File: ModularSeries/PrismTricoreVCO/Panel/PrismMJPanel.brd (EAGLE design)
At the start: 48.5 x 100 mm, 12 parts

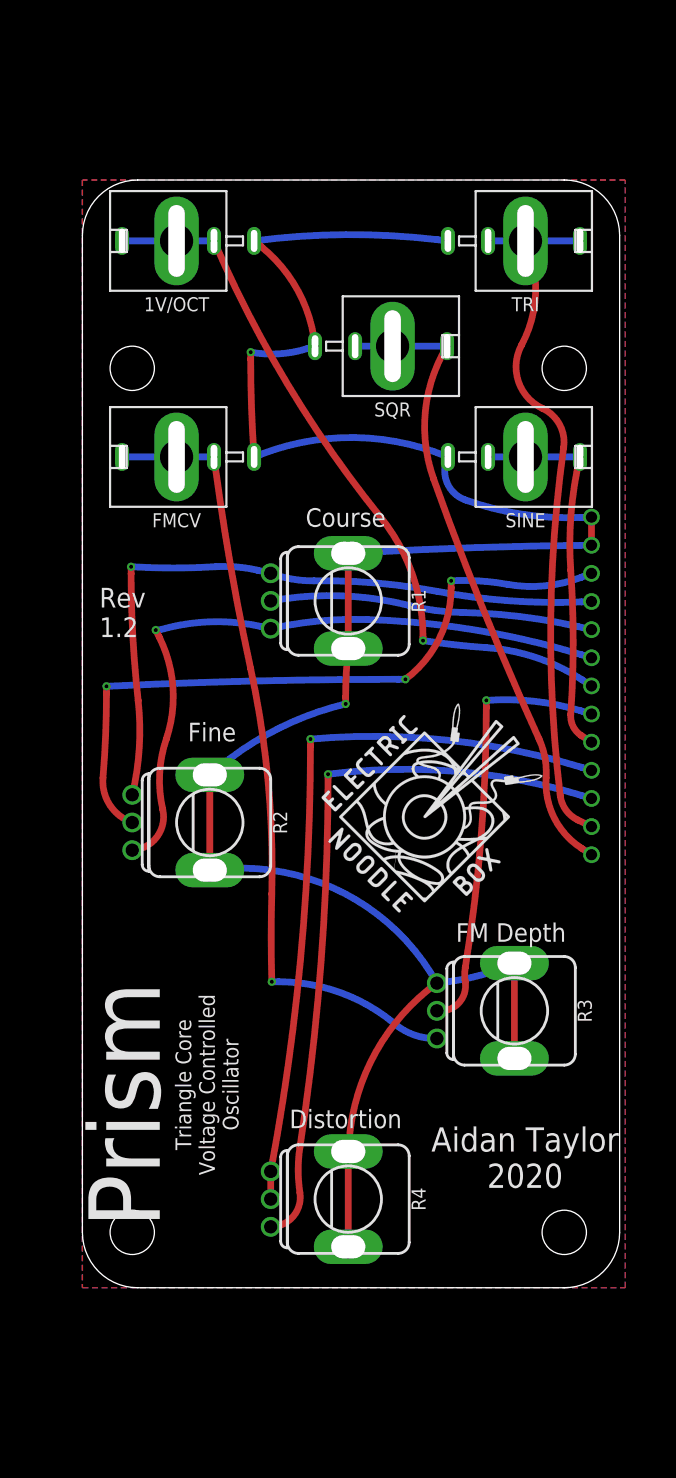
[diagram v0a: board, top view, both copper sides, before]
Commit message: Fields added and various updates to designs
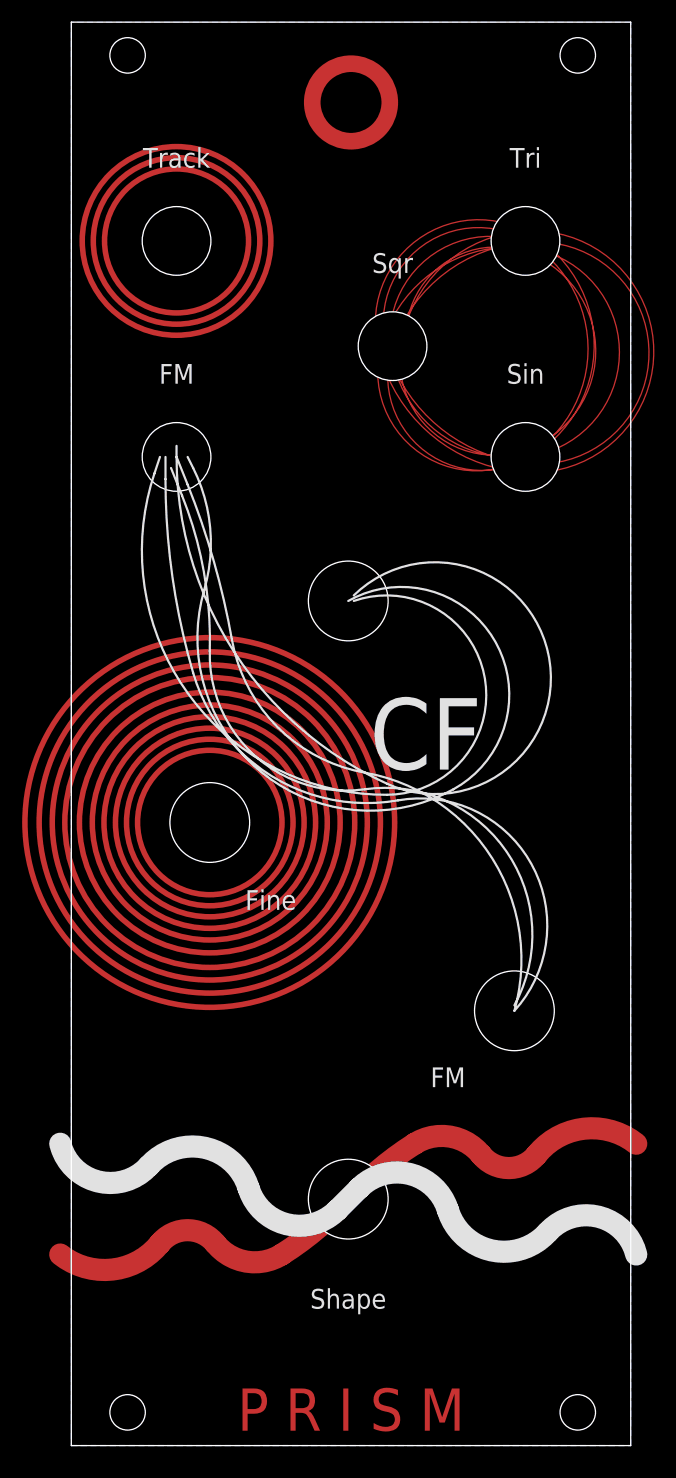
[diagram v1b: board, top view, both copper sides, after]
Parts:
- removed 1V/OCT, FMCV, SINE, SQR, TRI: COMBI-JACKCINCHNANA, ElectricNoodleBox:NEWCOMBOJACK_PANEL
- removed BOARD1: PRISM_LINK, ElectricNoodleBox:PRISM
- removed R1, R2, R3, R4: B100K, ElectricNoodleBox:ALPHA_RV09_9MMPOT
- removed U$1, U$2: (no value), ElectricNoodleBox:LOGO20X20
- added E$10: (no value), ElectricNoodleBox:LOGO20X20
- added E$6, E$7, E$8, E$9: (no value), ElectricNoodleBox:ALPHA9MM_POT_CUTOUT
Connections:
- removed net AGND: 1V/OCT.S, BOARD1.GNDA, BOARD1.GNDB, FMCV.S, R1.LUGL, R1.LUGR, R2.LUGL, R2.LUGR, R3.C1, R3.LUGL, R3.LUGR, R4.LUGL, R4.LUGR, SINE.S, SQR.S, TRI.S
- removed net N$1: 1V/OCT.CONN, 1V/OCT.T1, 1V/OCT.T2, BOARD1.CVA
- removed net N$10: BOARD1.SIN, SINE.CONN, SINE.T1, SINE.T2
- removed net N$11: BOARD1.TRI, TRI.CONN, TRI.T1, TRI.T2
- removed net N$12: BOARD1.SQR, SQR.CONN, SQR.T1, SQR.T2
- removed net N$2: BOARD1.F1, R1.C1, R2.C1
- removed net N$3: BOARD1.F3, R1.C3, R2.C3
- removed net N$4: BOARD1.F2, R1.C2
- removed net N$5: BOARD1.FINE, R2.C2
- removed net N$6: FMCV.CONN, FMCV.T1, FMCV.T2, R3.C3
- removed net N$7: BOARD1.CVB, R3.C2
- removed net N$8: BOARD1.DIST1, R4.C1, R4.C2
- removed net N$9: BOARD1.DIST2, R4.C3
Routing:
- net S$3: track 0.00 -> 325.8 mm
- net AGND: track 202.4 -> 0.00 mm, vias 2 -> 0
- net N$6: track 71.8 -> 0.00 mm, vias 1 -> 0
- net N$8: track 67.2 -> 0.00 mm, vias 1 -> 0
- net N$9: track 65.8 -> 0.00 mm, vias 1 -> 0
- net N$1: track 65.1 -> 0.00 mm, vias 1 -> 0
- net N$11: track 63.3 -> 0.00 mm
- net N$5: track 62.7 -> 0.00 mm, vias 3 -> 0
- net N$2: track 62.4 -> 0.00 mm, vias 1 -> 0
- net N$3: track 60.6 -> 0.00 mm, vias 1 -> 0
- net N$12: track 57.4 -> 0.00 mm
- net N$7: track 38.7 -> 0.00 mm, vias 1 -> 0
- net N$10: track 34.8 -> 0.00 mm
- net N$4: track 29.1 -> 0.00 mm
- net S$2: track 0.00 -> 28.0 mm
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- added copper zone on layer 16, net GND
- removed copper zone on layer 1, net AGND
- removed copper zone on layer 16, net AGND
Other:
- board size 48.5 x 100 mm -> 50.5 x 128.5 mm
- board text added: "CF"
- board text added: "F L U X E S"
- board text added: "FM"
- board text added: "O R B I T S"
- board text added: "P R I S M"
- board text added: "Shape"
- board text added: "Sin"
- board text added: "Sqr"
- board text added: "T E N S I O N S"
- board text added: "Track"
- board text added: "Tri"
- board text removed: "Aidan Taylor 2020"
- board text removed: "Course"
- board text removed: "Distortion"
- board text removed: "FM Depth"
- board text removed: "Prism"
- board text removed: "Rev 1.2"
- board text removed: "Triangle Core Voltage Controlled Oscillator"
